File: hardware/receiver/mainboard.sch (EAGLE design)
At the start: 5 parts, among them U1 ATMEGA328P_TQFP, U2 RFM69HCW

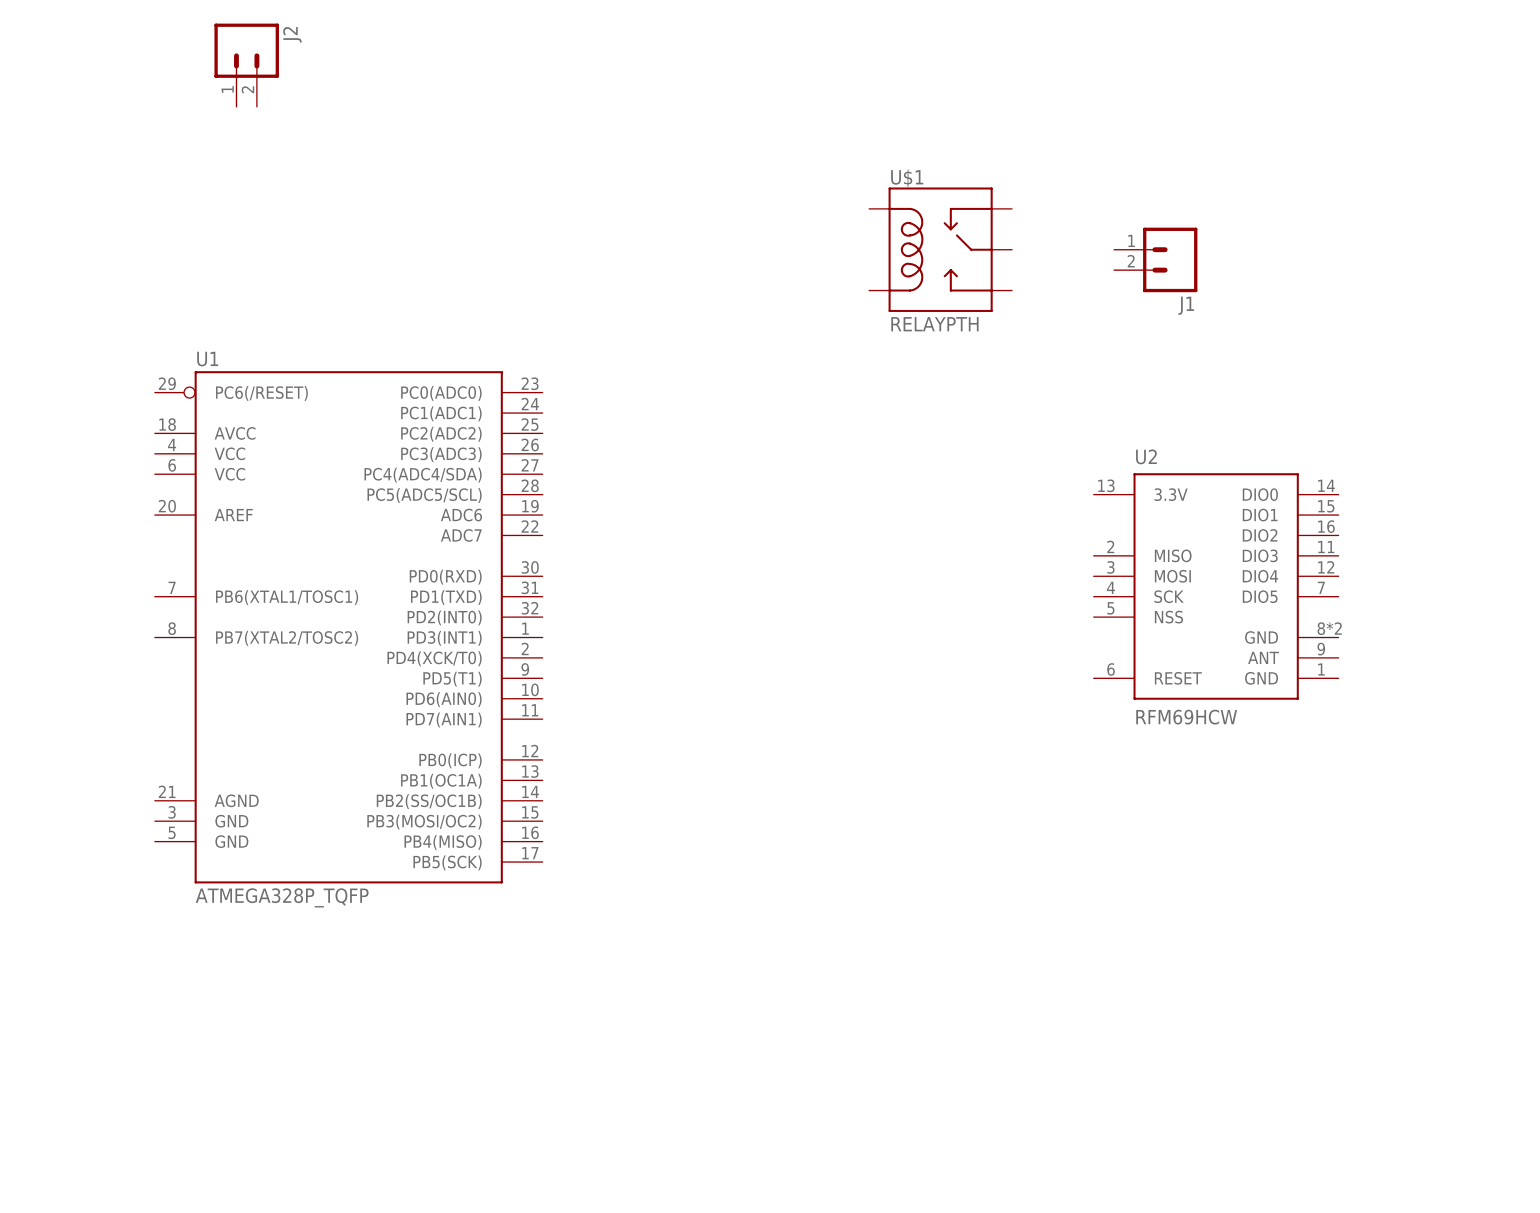
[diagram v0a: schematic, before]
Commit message: Preliminary schematic
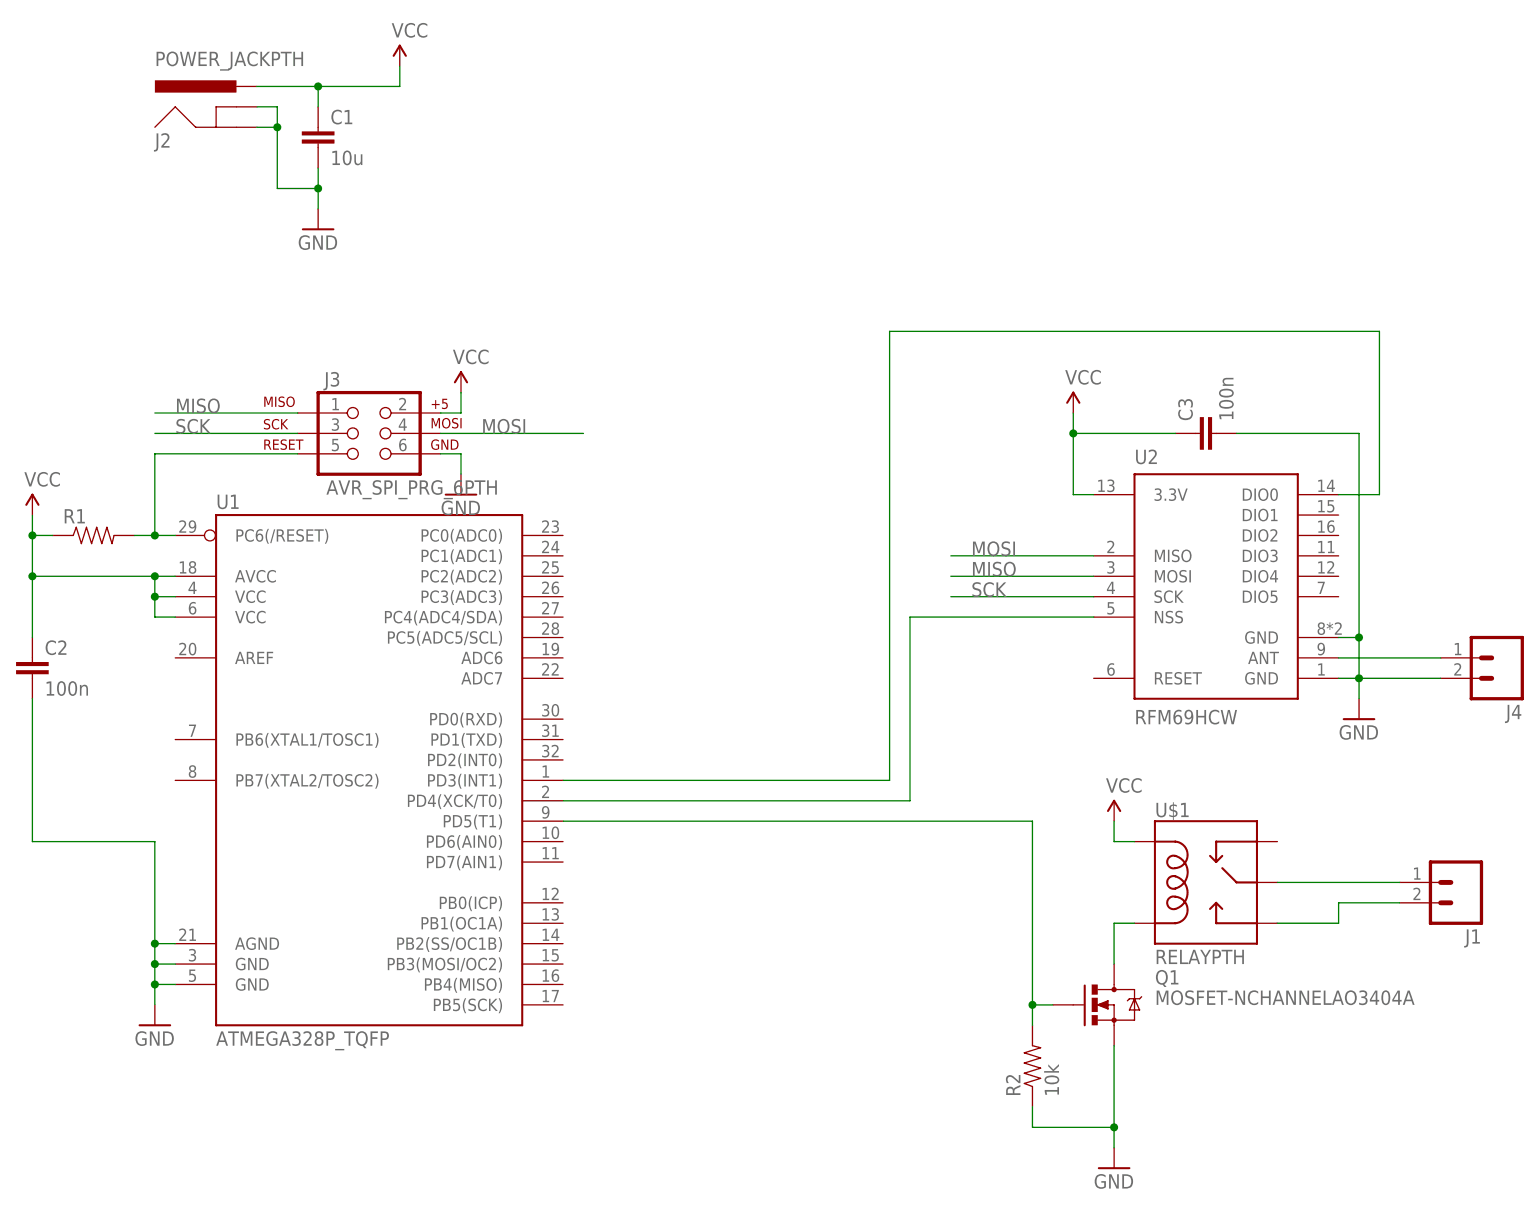
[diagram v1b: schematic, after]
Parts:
- added C1: 10u, SparkFun-Passives:CAP1206
- added C2, C3: 100n, SparkFun-Passives:CAP0603-CAP
- added J3: AVR_SPI_PRG_6PTH, SparkFun-Connectors:AVR_SPI_PRG_6PTH
- added J4: (no value), SparkFun-Connectors:M02PTH
- added Q1: MOSFET-NCHANNELAO3404A, SparkFun-DiscreteSemi:MOSFET-NCHANNELAO3404A
- added R1: (no value), SparkFun-Passives:RESISTOR0603-RES
- added R2: 10k, SparkFun-Passives:RESISTOR0603-RES
- J2: value (none) -> POWER_JACKPTH; device SparkFun-Connectors:M025MM -> SparkFun-Connectors:POWER_JACKPTH
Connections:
- new net GND: C1.2, C2.2, C3.2, J2.GND, J2.GNDBREAK, J3.6, J4.2, Q1.S, R2.1, U1.AGND, U1.GND@3, U1.GND@5, U2.GND@1, U2.GND@2
- new net MISO: J3.1, U2.MOSI
- new net MOSI: J3.4, U2.MISO
- new net N$1: U1.PD4(XCK/T0), U2.NSS
- new net N$2: J3.5, R1.2, U1.PC6(/RESET)
- new net N$3: U1.PD3(INT1), U2.DIO0
- new net N$4: J4.1, U2.ANT
- new net N$5: J1.1, U$1.MAIN
- new net N$6: J1.2, U$1.NO
- new net N$7: Q1.D, U$1.COIL2
- new net N$8: Q1.G, R2.2, U1.PD5(T1)
- new net SCK: J3.3, U2.SCK
- new net VCC: C1.1, C2.1, C3.1, J2.PWR, J3.2, R1.1, U$1.COIL1, U1.AVCC, U1.VCC@4, U1.VCC@6, U2.3.3V
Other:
- moved on the sheet: J1, J2, U$1, U1
